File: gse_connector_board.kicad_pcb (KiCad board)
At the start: 2 copper layers, 50 x 20 mm, 19 parts, among them J1 arming_connector, J2 gse_com_connector, J3 chg_connector, U4 L7805, U7 ISO1044BD, U9 MCP2562-E-SN

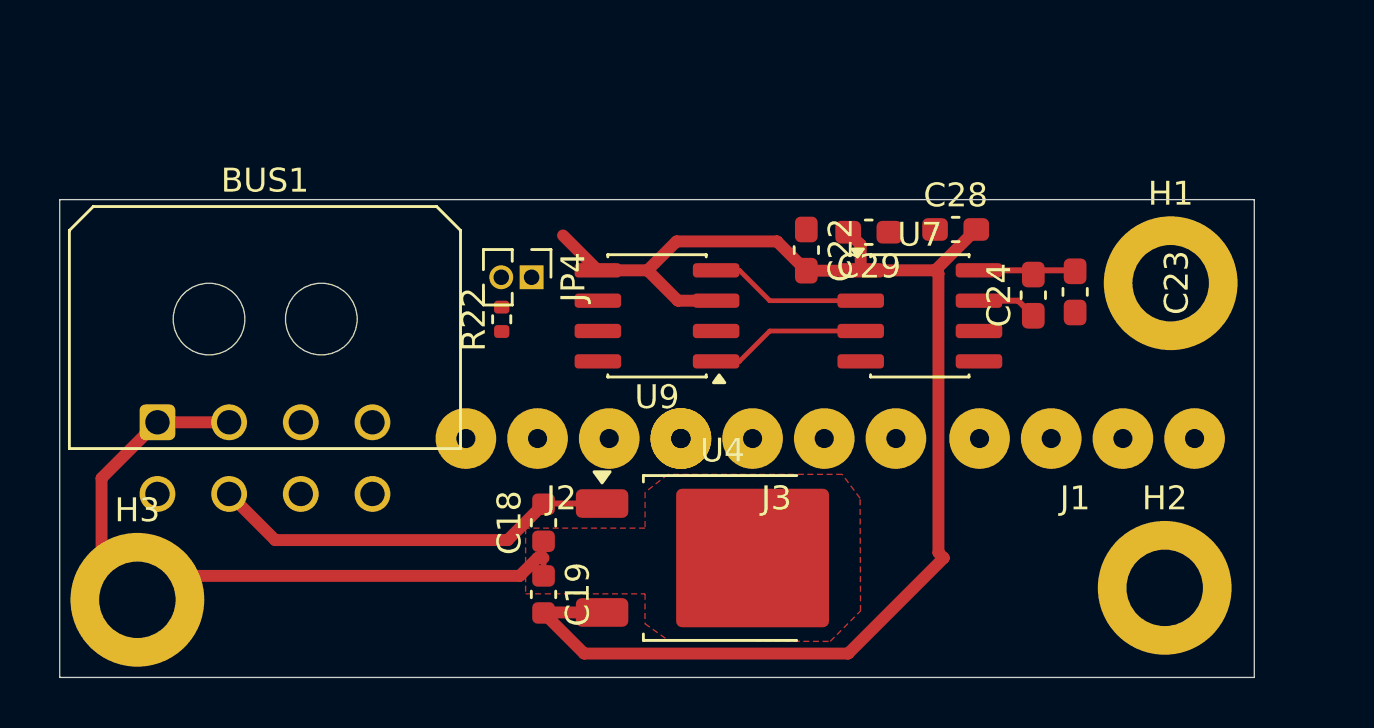
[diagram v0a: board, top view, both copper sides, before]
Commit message: wip
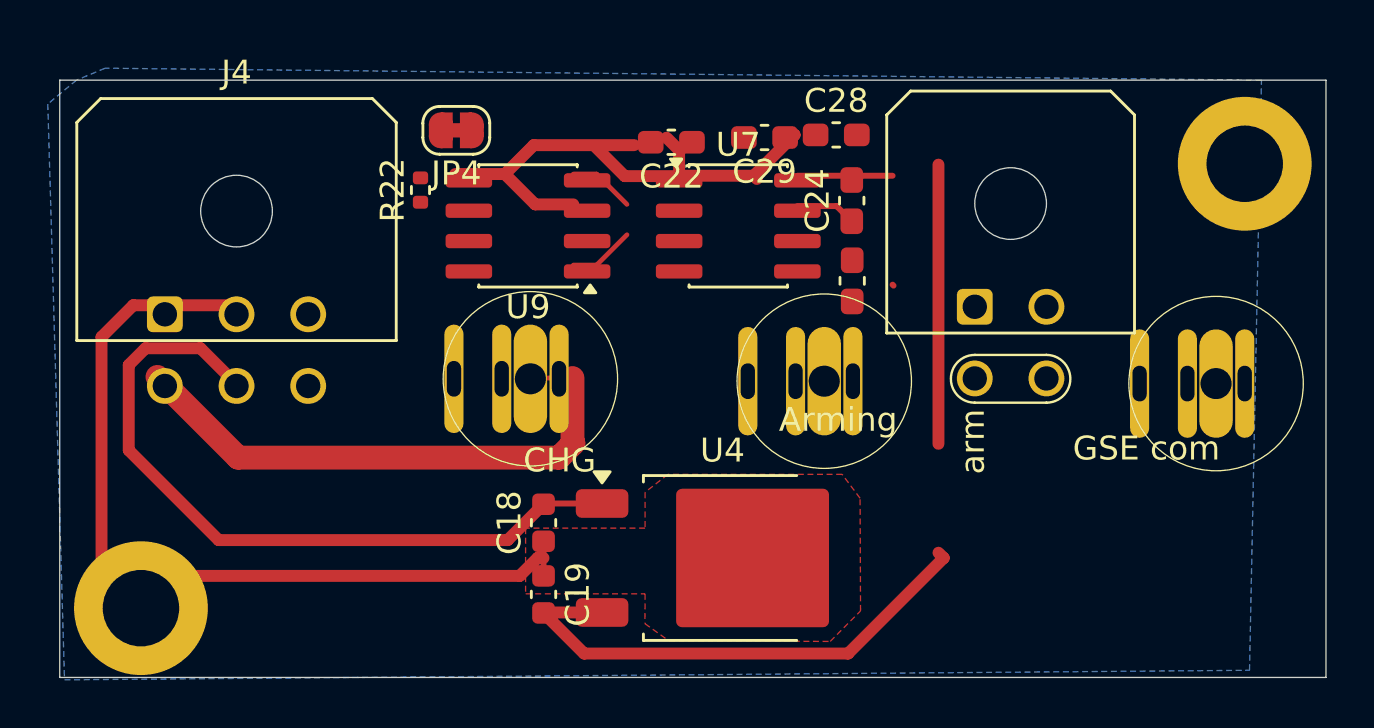
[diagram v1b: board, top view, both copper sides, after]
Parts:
- removed BUS1: 43045-0800, Connector_Molex:Molex_Micro-Fit_3.0_43045-0800_2x04_P3.00mm_Horizontal
- removed H3: MountingHole_Pad, MountingHole:MountingHole_3.2mm_M3_DIN965_Pad
- added J4: Conn_02x03_Top_Bottom, Connector_Molex:Molex_Micro-Fit_3.0_43045-0600_2x03_P3.00mm_Horizontal, F.Cu at (121.4, 66.3)
- added J5: Conn_02x02_Top_Bottom, Connector_Molex:Molex_Micro-Fit_3.0_43045-0400_2x02_P3.00mm_Horizontal, F.Cu at (155.3, 66.0)
- JP4: footprint Connector_PinHeader_1.27mm:PinHeader_1x02_P1.27mm_Vertical -> Jumper:SolderJumper-2_P1.3mm_Bridged_RoundedPad1.0x1.5mm
- moved H2 42.9 mm to (120.4, 78.6)
- moved J2 11.3 mm to (149.0, 72.1)
- moved J3 10.6 mm to (136.7, 72.0)
- moved C23 9.34 mm to (150.2, 64.9)
- moved C24 8.57 mm to (150.2, 61.5)
- moved U7 8.48 mm to (145.4, 62.6)
- moved C22 7.23 mm to (142.6, 59.1), turned to 180 degrees
- moved JP4 6.91 mm to (133.6, 58.6), turned to 180 degrees
- moved U9 6.58 mm to (136.6, 62.6)
- moved R22 6.39 mm to (132.1, 61.1)
- moved C28 6.38 mm to (149.5, 58.8)
- moved J1 6.33 mm to (165.4, 72.2)
- moved C29 5.90 mm to (146.5, 58.9)
- moved H1 5.88 mm to (166.6, 60.0)
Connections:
- J1 pad 1: supply -> main_voltage
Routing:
- net CHG: track 0.00 -> 23.0 mm
- net main_voltage: track 17.0 -> 30.6 mm
- net GND: track 30.8 -> 36.3 mm
- net Net-(U7-TXD): track 6.58 -> 2.77 mm
- net Net-(U7-RXD): track 6.58 -> 2.77 mm
- net +5V: track 58.6 -> 56.5 mm
- added copper zone on B.Cu, net GND
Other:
- board size 50 x 20 mm -> 53 x 25 mm
- board text added: "Arming"
- board text added: "CHG"
- board text added: "GSE com"
- board text added: "arm"
